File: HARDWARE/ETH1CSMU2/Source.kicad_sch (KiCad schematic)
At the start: 99 parts, among them Q901 FDV301N, U901 DAC8565ICPW, U902 AD9834BRUZ, U903 MC74AC161DR2G, U904 MAX6102EUR, U905 MAX5217GUA+, U906 SN74AHC1G14DBVT, U907 OPA2141AID, U908 MC74AC161DR2G, U909 SN74AUP1G79DCKR, U910 LM7171BIM, U911 OPA141AID, U912 DG409DY+, U913 AD5322ARMZ, U914 LT1790BCS6-2.5, U915 TL071CDR, U916 LM7171BIM, X901 830208220601

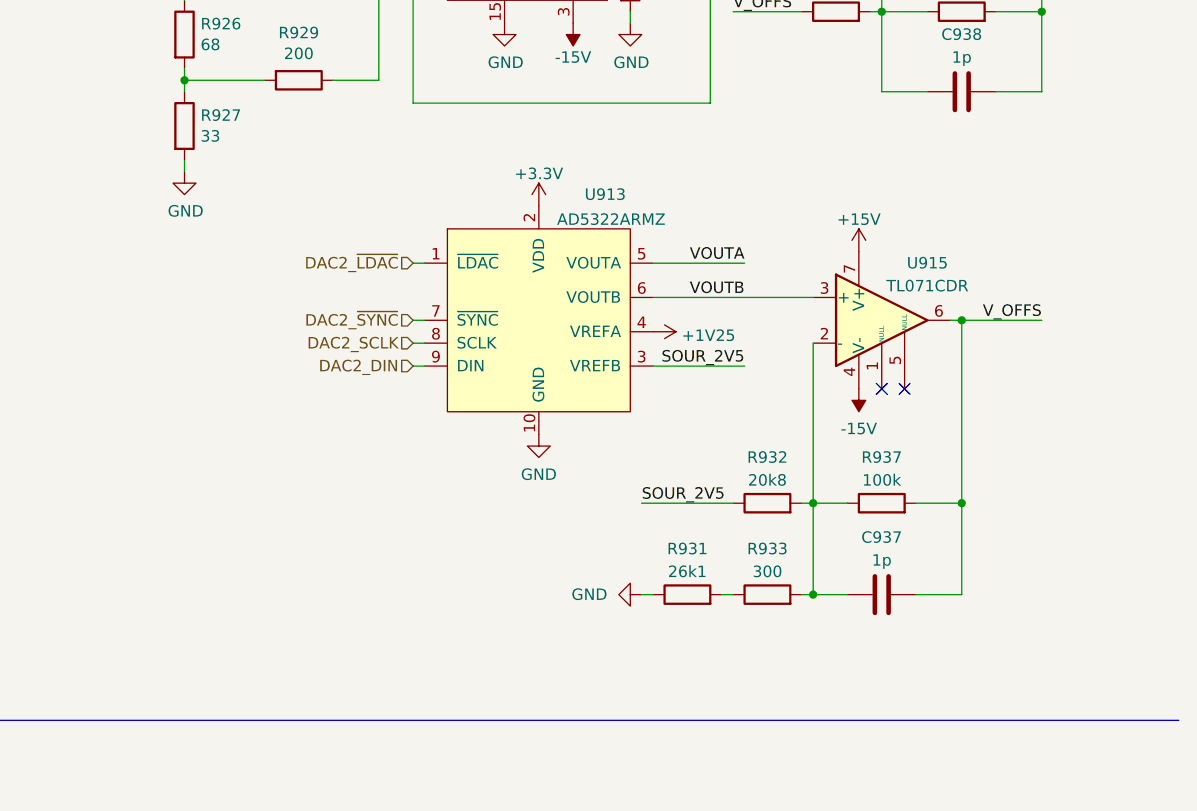
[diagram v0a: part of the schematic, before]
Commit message: Software development
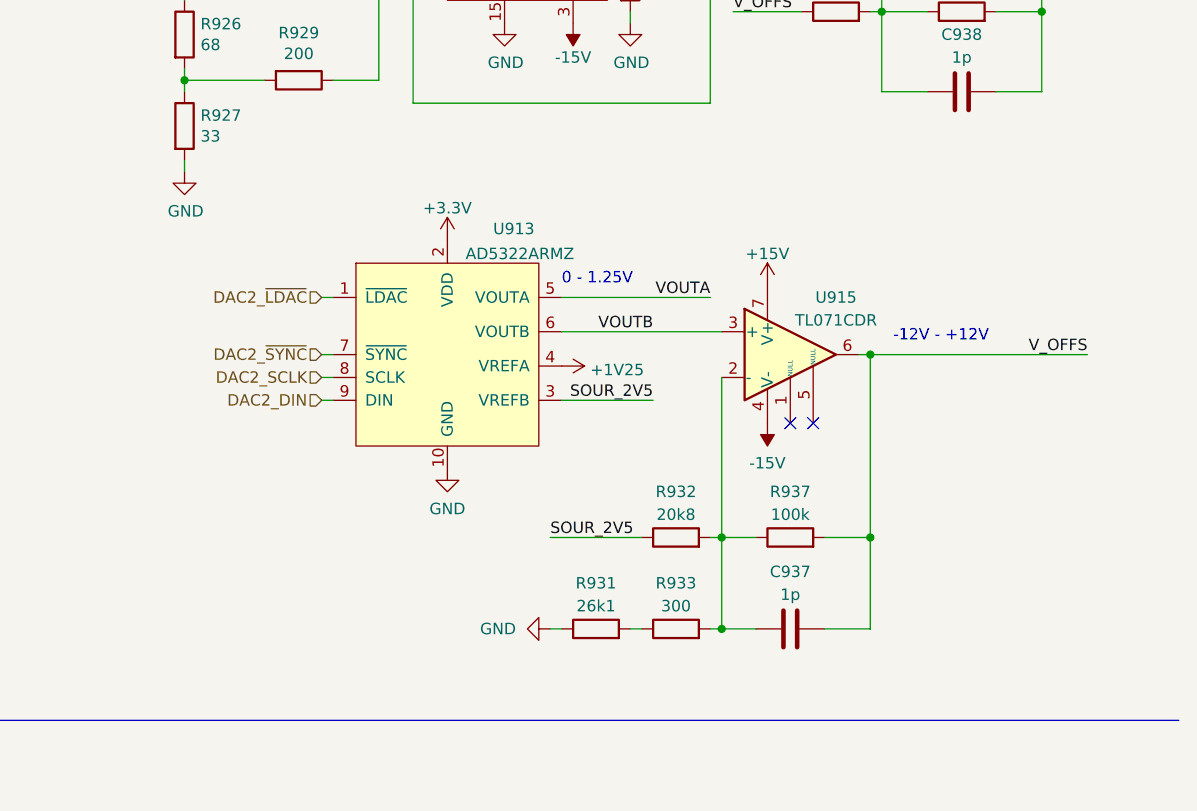
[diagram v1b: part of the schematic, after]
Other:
- note added: "-12V - +12V"
- note added: "0 - 1.25V"
- moved on the sheet: C937, R931, R932, R933, R937, U913, U915
